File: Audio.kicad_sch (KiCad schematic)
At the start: 20 parts, among them CN2 PJ-3537S, U3 SGTL5000XNAA3R2, U8 PCM1807PW

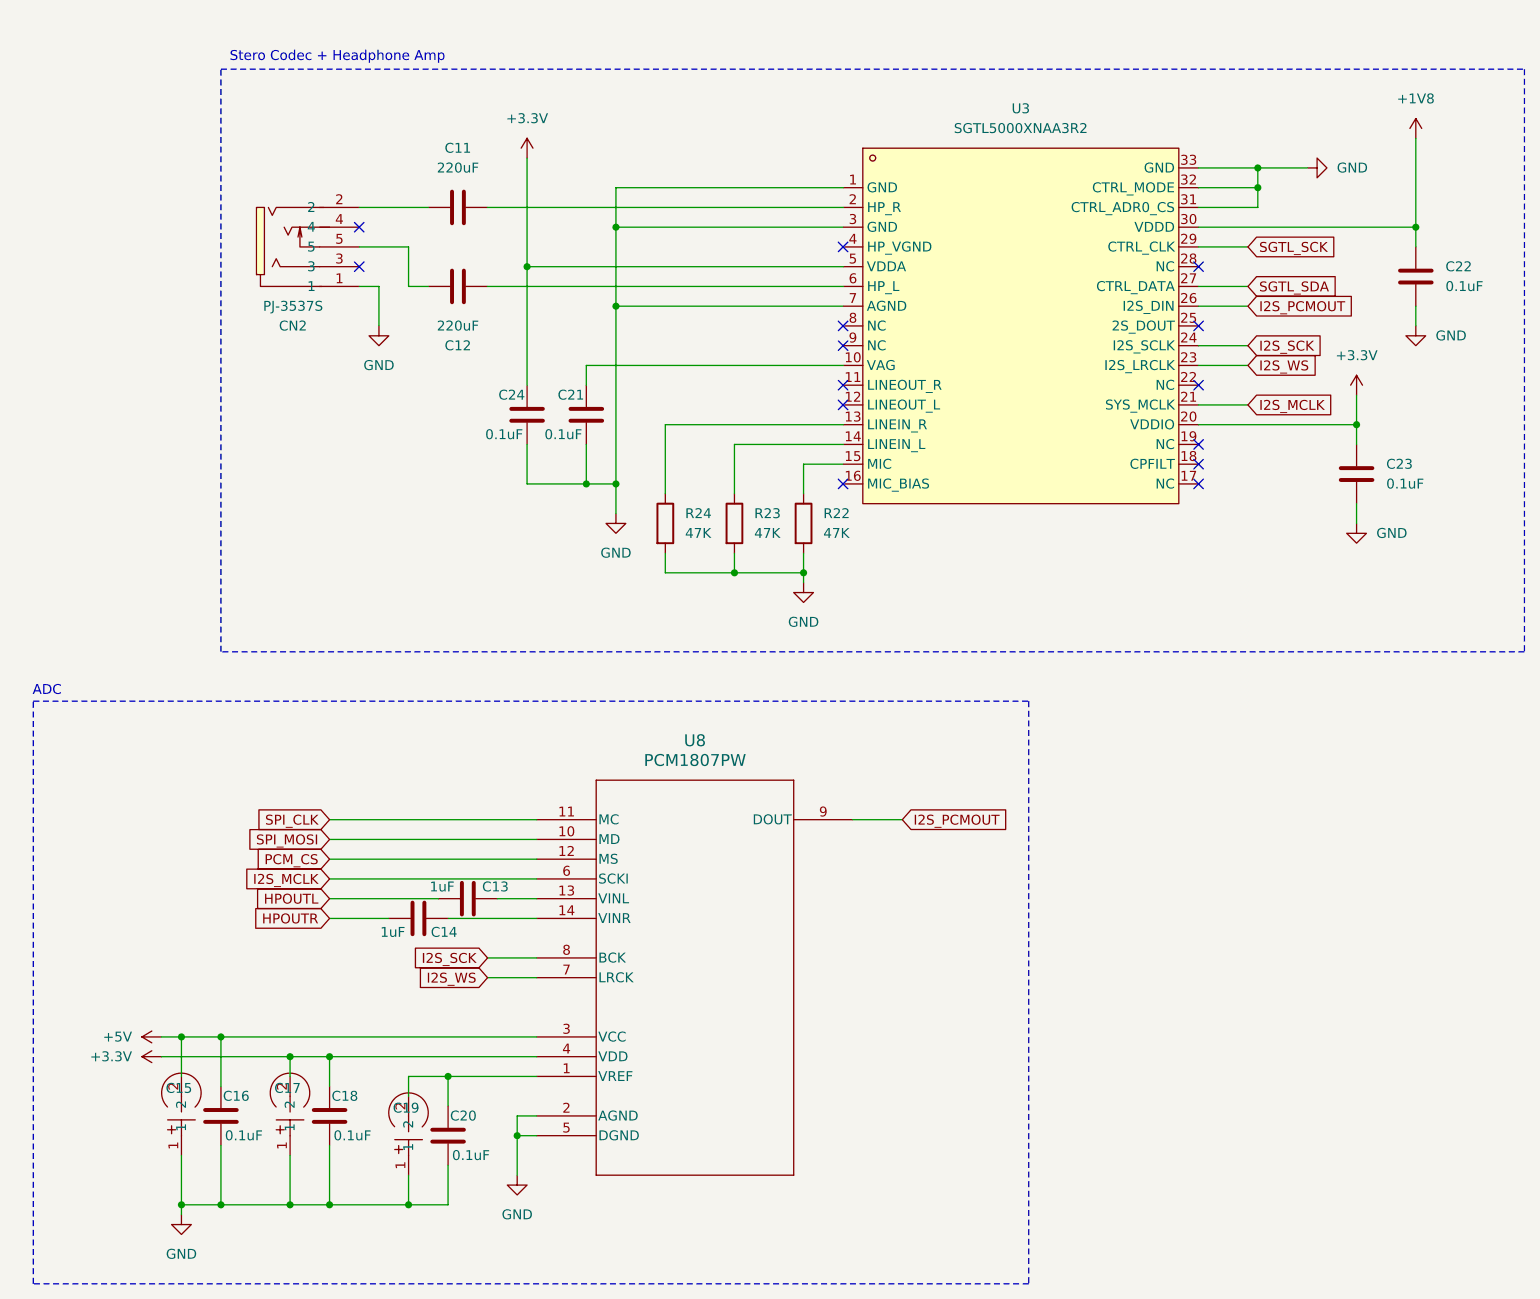
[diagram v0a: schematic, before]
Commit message: power changes for v3s, cleanup
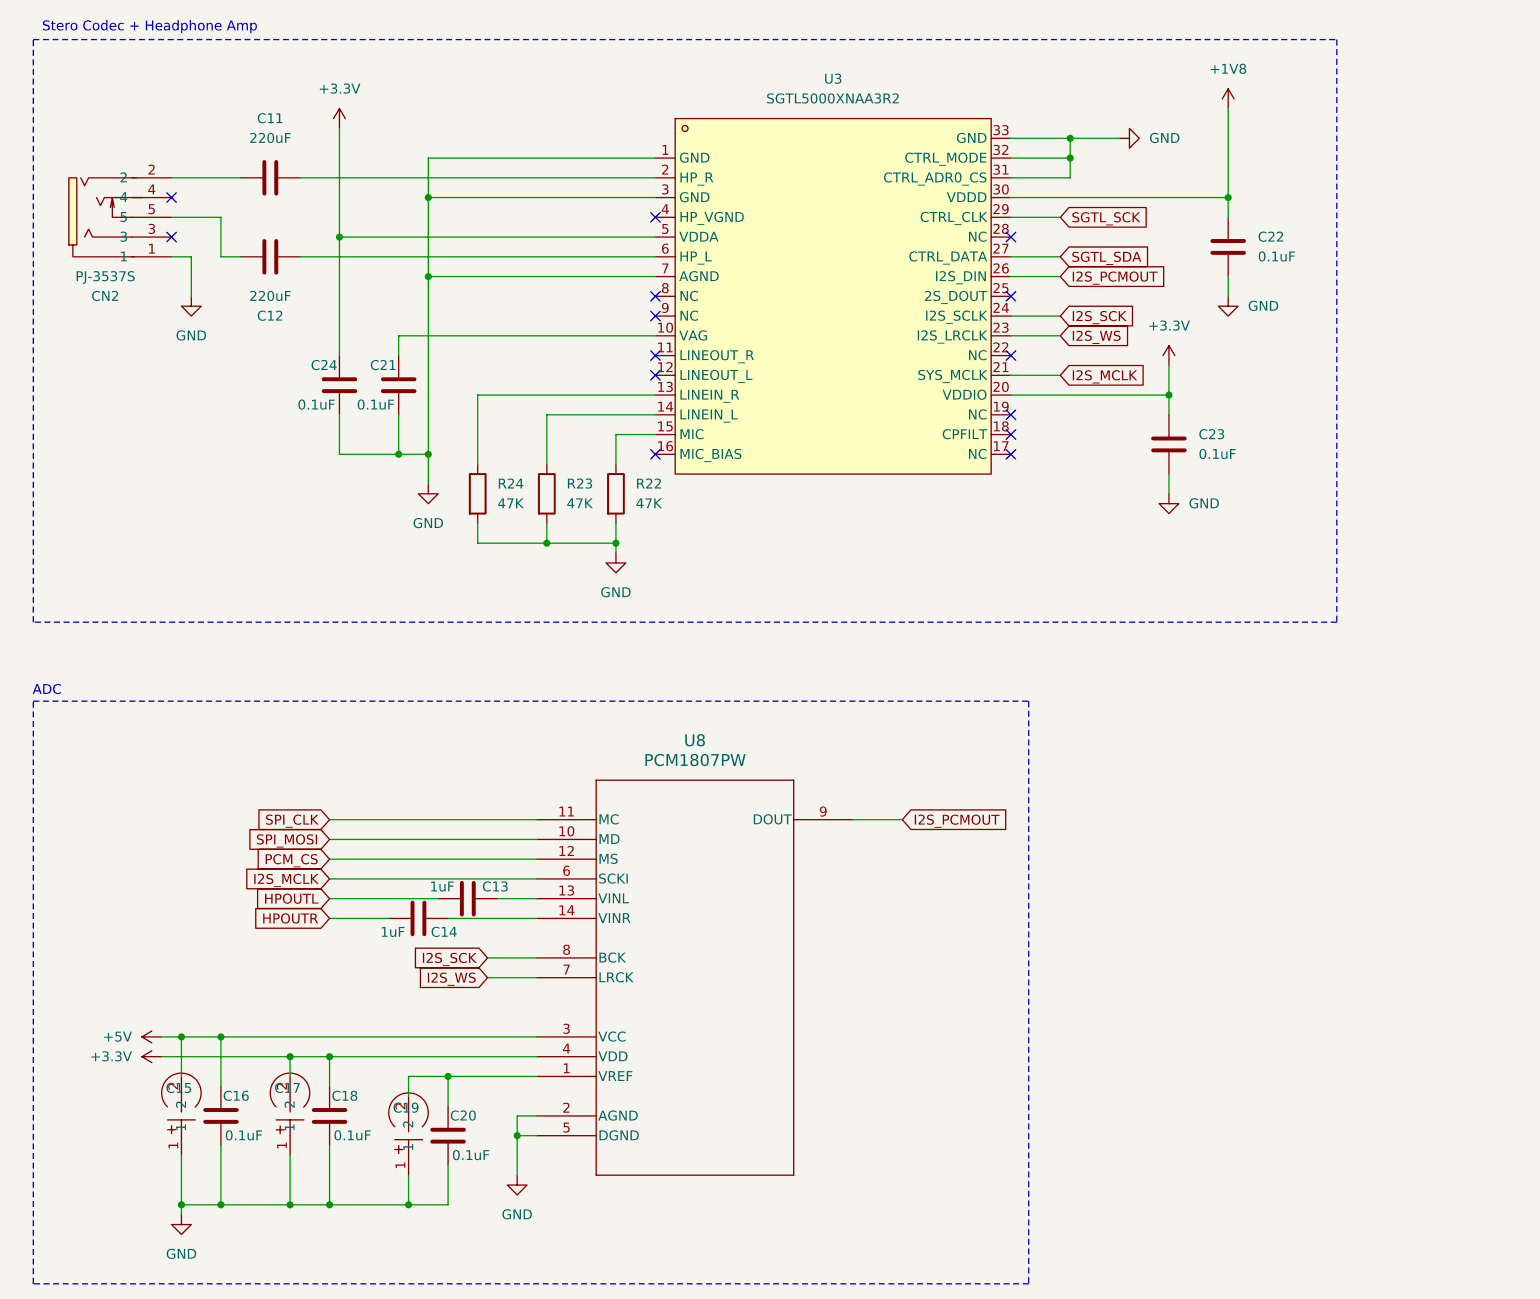
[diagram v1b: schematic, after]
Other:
- title: (none) -> iPodClone
- moved on the sheet: C11, C12, C21, C22, C23, C24, CN2, R22, R23, R24, U3
